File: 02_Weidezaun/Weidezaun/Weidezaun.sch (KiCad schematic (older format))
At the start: 8 parts, among them J1 Screw_Terminal_01x02, J2 Screw_Terminal_01x02, Q1 2N7000

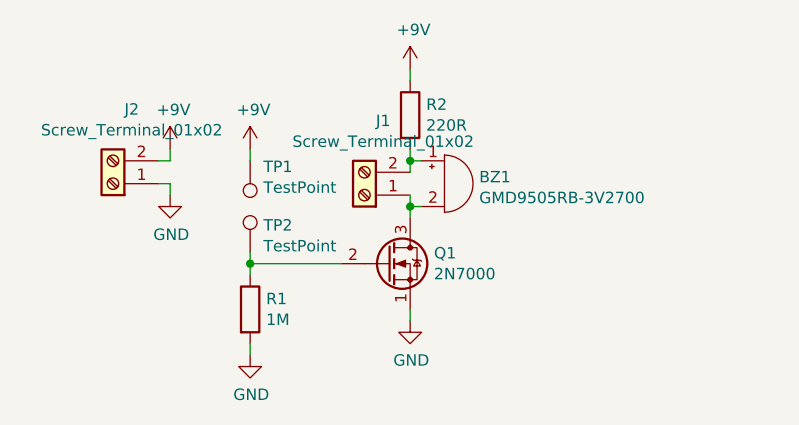
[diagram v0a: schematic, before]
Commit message: review
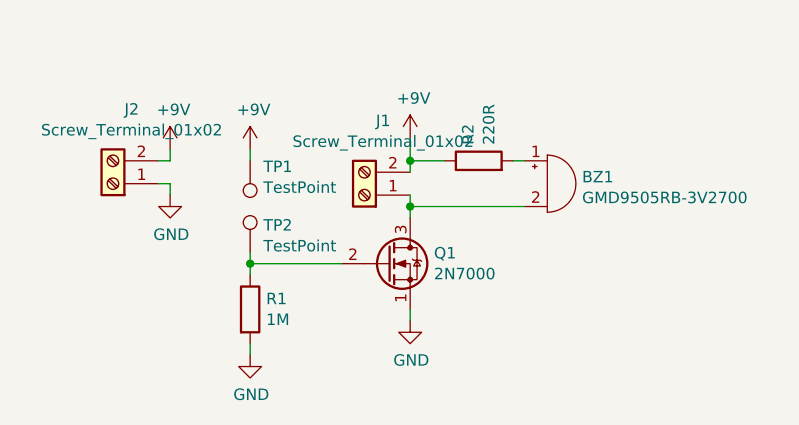
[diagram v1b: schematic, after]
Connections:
- net +9V: now also J1.2 (Pin_2)
- net at BZ1.1 (-), R2.2: no longer J1.2 (Pin_2)
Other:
- moved on the sheet: BZ1, R2
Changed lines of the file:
@@
 L Device:Buzzer BZ1
 U 1 1 61606991
-P 5000 3250
-F 0 "BZ1" H 5152 3279 50  0000 L CNN
-F 1 "GMD9505RB-3V2700" H 5152 3188 50  0000 L CNN
-F 2 "Buzzer_Beeper:Buzzer_TDK_PS1240P02BT_D12.2mm_H6.5mm" V 4975 3350 50  0001 C CNN
-F 3 "~" V 4975 3350 50  0001 C CNN
-	1    5000 3250
+P 5450 3250
+F 0 "BZ1" H 5602 3279 50  0000 L CNN
+F 1 "GMD9505RB-3V2700" H 5602 3188 50  0000 L CNN
+F 2 "Buzzer_Beeper:Buzzer_TDK_PS1240P02BT_D12.2mm_H6.5mm" V 5425 3350 50  0001 C CNN
+F 3 "~" V 5425 3350 50  0001 C CNN
+	1    5450 3250
 	1    0    0    -1
 $EndComp
-Wire Wire Line
-	4900 3350 4850 3350
 Wire Wire Line
 	4850 3350 4850 3400
@@
 L Device:R R2
 U 1 1 61607437
-P 4850 2950
-F 0 "R2" H 4920 2996 50  0000 L CNN
-F 1 "220R" H 4920 2905 50  0000 L CNN
-F 2 "Resistor_THT:R_Axial_DIN0204_L3.6mm_D1.6mm_P7.62mm_Horizontal" V 4780 2950 50  0001 C CNN
-F 3 "~" H 4850 2950 50  0001 C CNN
-	1    4850 2950
-	1    0    0    -1
+P 5150 3150
+F 0 "R2" H 5220 3196 50  0000 L CNN
+F 1 "220R" H 5220 3105 50  0000 L CNN
+F 2 "Resistor_THT:R_Axial_DIN0204_L3.6mm_D1.6mm_P7.62mm_Horizontal" V 5080 3150 50  0001 C CNN
+F 3 "~" H 5150 3150 50  0001 C CNN
+	1    5150 3150
+	0    -1   -1   0
 $EndComp
-Wire Wire Line
-	4850 3100 4850 3150
-Wire Wire Line
-	4850 3150 4900 3150
-Wire Wire Line
-	4850 2750 4850 2800
 $Comp
 L Connector:Screw_Terminal_01x02 J1
@@
 L power:+9V #PWR06
 U 1 1 616026A6
-P 4850 2750
-F 0 "#PWR06" H 4850 2600 50  0001 C CNN
-F 1 "+9V" H 4865 2923 50  0000 C CNN
-F 2 "" H 4850 2750 50  0001 C CNN
-F 3 "" H 4850 2750 50  0001 C CNN
-	1    4850 2750
+P 4850 3050
+F 0 "#PWR06" H 4850 2900 50  0001 C CNN
+F 1 "+9V" H 4865 3223 50  0000 C CNN
+F 2 "" H 4850 3050 50  0001 C CNN
+F 3 "" H 4850 3050 50  0001 C CNN
+	1    4850 3050
 	1    0    0    -1
 $EndComp
@@
 Wire Wire Line
 	3800 3250 3800 3300
+Wire Wire Line
+	4850 3350 5350 3350
+Wire Wire Line
+	5350 3150 5300 3150
+Wire Wire Line
+	4850 3150 5000 3150
+Wire Wire Line
+	4850 3050 4850 3150
 $EndSCHEMATC

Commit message: changed footprint
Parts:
- Q1: footprint Package_TO_SOT_THT:TO-92_Inline -> Package_TO_SOT_THT:TO-92_Inline_Wide
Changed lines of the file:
@@
 F 0 "Q1" H 4954 3646 50  0000 L CNN
 F 1 "2N7000" H 4954 3555 50  0000 L CNN
-F 2 "Package_TO_SOT_THT:TO-92_Inline" H 4950 3525 50  0001 L CIN
+F 2 "Package_TO_SOT_THT:TO-92_Inline_Wide" H 4950 3525 50  0001 L CIN
 F 3 "https://www.onsemi.com/pub/Collateral/NDS7002A-D.PDF" H 4750 3600 50  0001 L CNN
 	1    4750 3600
